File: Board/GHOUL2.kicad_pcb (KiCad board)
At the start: 2 copper layers, 106.7 x 73.7 mm, 16 parts, among them J1 Conn_01x02, Q1 IRF540N, Q2 IRF540N, U1 Teensy3.5_All_Pins, U10 GHOULIMU, U2 LM7805_TO220, U3 BMP280, U4 Feedback_Serv, U5 LM1084-ADJ, U6 NichromeConnector, U7 Ultimate_GPS_Breakout_v3, U8 Xbee, U9 NichromeConnector

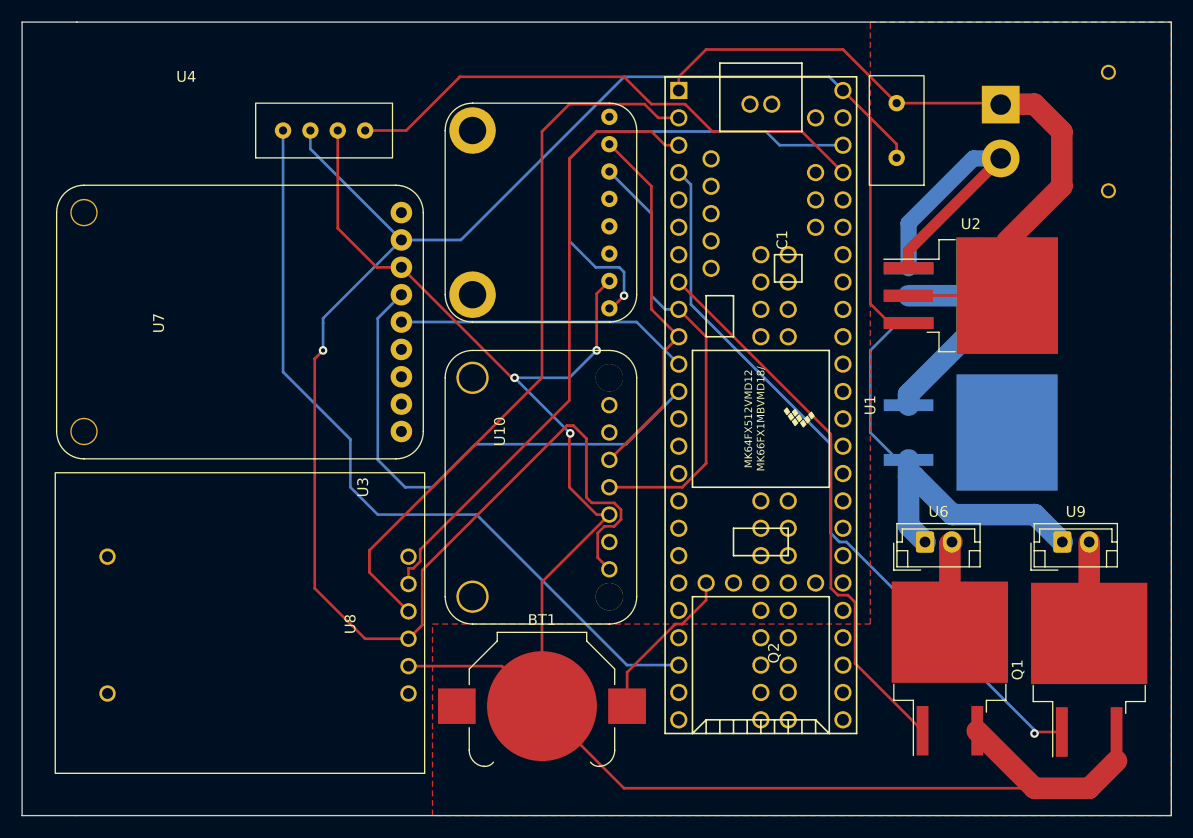
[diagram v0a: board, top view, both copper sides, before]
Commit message: sometimes the fastest way to get to the end is to throw everything out and start over
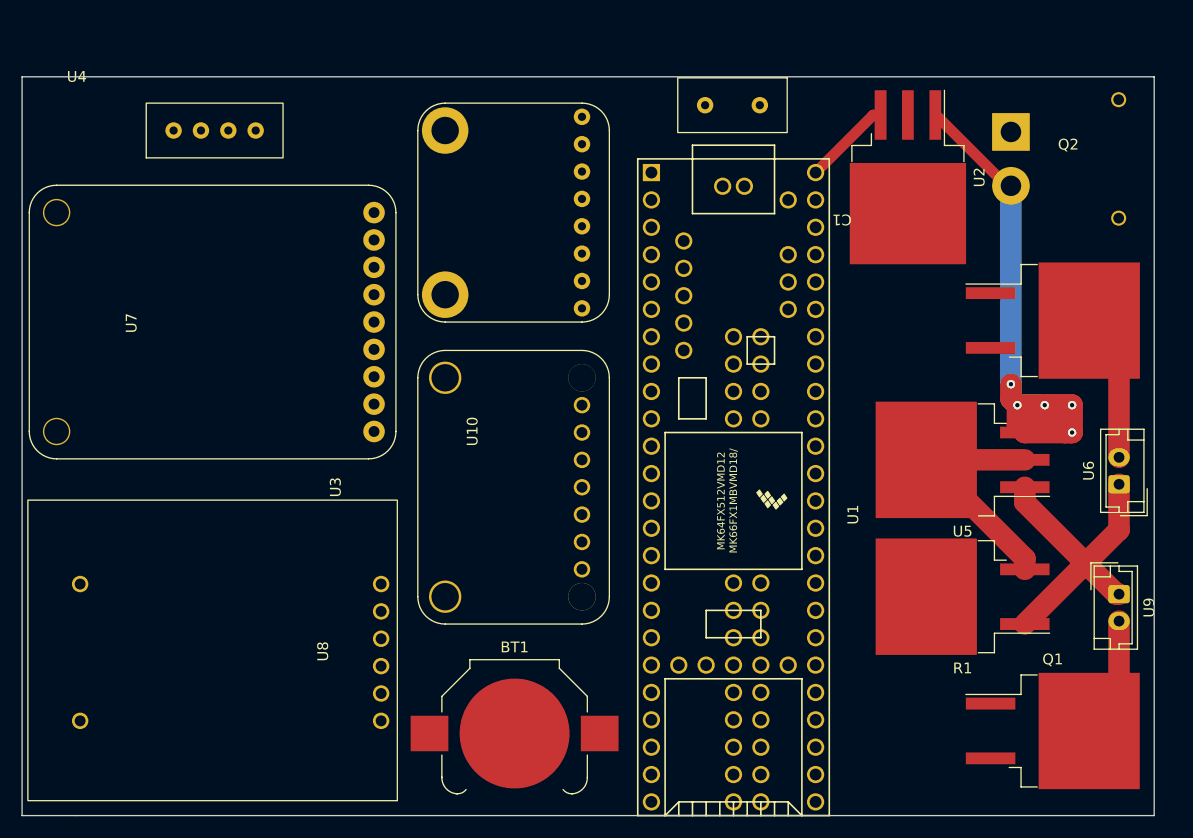
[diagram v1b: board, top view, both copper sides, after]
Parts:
- R1, U5: moved to F.Cu
- moved Q2 33.7 mm to (189.7, 91.2), turned to 0 degrees
- moved U6 18.8 mm to (195.8, 106.4), turned to 90 degrees
- moved C1 16.1 mm to (165.0, 68.7), turned to 180 degrees
- moved R1 15.3 mm to (181.3, 116.8), turned to 180 degrees
- moved U5 15.3 mm to (181.3, 104.1), turned to 180 degrees
- moved U2 12.4 mm to (176.2, 77.9), turned to -90 degrees
- moved U4 10.2 mm to (105.5, 76.1)
- moved U1 8.03 mm to (160.0, 106.7)
- moved U9 7.16 mm to (195.8, 116.6), turned to -90 degrees
- moved Q1 6.61 mm to (189.7, 129.3), turned to 0 degrees
- moved BT1 3.59 mm to (139.7, 129.5)
- moved U8 3.59 mm to (128.8, 135.8)
- moved J1 2.71 mm to (185.8, 73.7)
- moved U7 2.54 mm to (128.7, 104.0)
- moved U10 2.54 mm to (148.5, 91.3)
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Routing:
- net GND: track 235.9 -> 0.00 mm, vias 3 -> 0
- net 5v pwr: track 182.4 -> 8.24 mm, vias 1 -> 0
- net Net-(U1-Pad22): track 73.0 -> 0.00 mm
- net Nic2: track 68.7 -> 0.00 mm, vias 1 -> 0
- net Net-(U1-Pad2): track 67.0 -> 0.00 mm
- net Net-(U1-Pad3): track 57.7 -> 0.00 mm
- net Nic1: track 51.6 -> 0.00 mm
- net Feedback: track 50.1 -> 0.00 mm
- net Net-(U1-Pad12): track 48.9 -> 0.00 mm
- net Net-(U1-Pad51): track 44.9 -> 0.00 mm, vias 1 -> 0
- net Net-(U1-Pad9): track 41.5 -> 0.00 mm
- net Net-(U1-Pad10): track 34.6 -> 0.00 mm
- net Vin: track 29.0 -> 60.9 mm, vias 0 -> 5
- net Net-(U1-Pad11): track 27.4 -> 0.00 mm
- net Net-(BT1-Pad1): track 14.8 -> 0.00 mm
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- removed copper zone on F.Cu, net GND
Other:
- board size 106.7 x 73.7 mm -> 105.1 x 68.6 mm

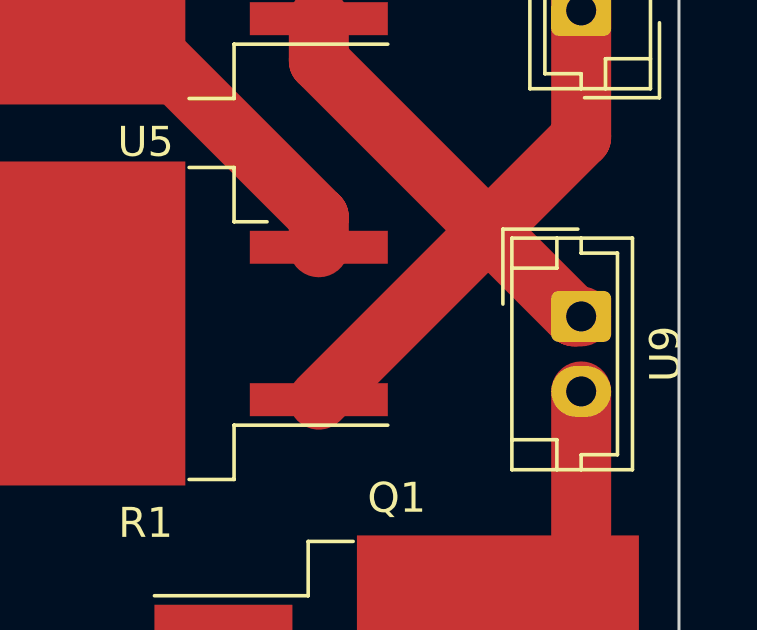
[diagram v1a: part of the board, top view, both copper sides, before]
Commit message: fixed some routing
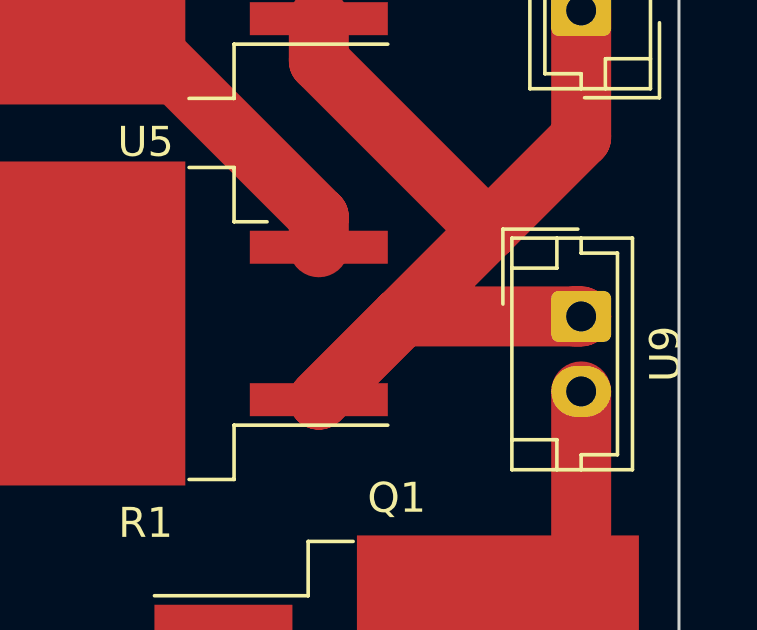
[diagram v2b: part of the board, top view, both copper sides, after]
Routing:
- net Net-(R1-Pad1): track 30.3 -> 36.1 mm
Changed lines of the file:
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@@
   (segment (start 195.81 103.905) (end 195.81 93.975) (width 2) (layer "F.Cu") (net 24))
   (segment (start 195.81 93.975) (end 193.04 91.205) (width 0.25) (layer "F.Cu") (net 24))
+  (segment (start 189.84 116.605) (end 195.81 116.605) (width 2) (layer "F.Cu") (net 25))
   (segment (start 195.81 110.635) (end 195.81 106.405) (width 2) (layer "F.Cu") (net 25))
   (segment (start 195.58 116.605) (end 195.81 116.605) (width 2) (layer "F.Cu") (net 25))
-  (segment (start 192.71 113.735) (end 195.58 116.605) (width 2) (layer "F.Cu") (net 25))
   (segment (start 187.065 106.68) (end 187.065 108.09) (width 2) (layer "F.Cu") (net 25))
   (segment (start 187.065 108.09) (end 192.71 113.735) (width 2) (layer "F.Cu") (net 25))
+  (segment (start 187.065 119.38) (end 192.71 113.735) (width 2) (layer "F.Cu") (net 25))
+  (segment (start 187.065 119.38) (end 189.84 116.605) (width 2) (layer "F.Cu") (net 25))
   (segment (start 192.71 113.735) (end 195.81 110.635) (width 2) (layer "F.Cu") (net 25))
-  (segment (start 187.065 119.38) (end 192.71 113.735) (width 2) (layer "F.Cu") (net 25))
   (segment (start 173.67 72.13) (end 172.98 72.13) (width 1) (layer "F.Cu") (net 45))
   (segment (start 172.98 72.13) (end 167.64 77.47) (width 1) (layer "F.Cu") (net 45))
